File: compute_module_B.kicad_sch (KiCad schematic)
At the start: 2 parts, among them J12 HDMI_A_1.4

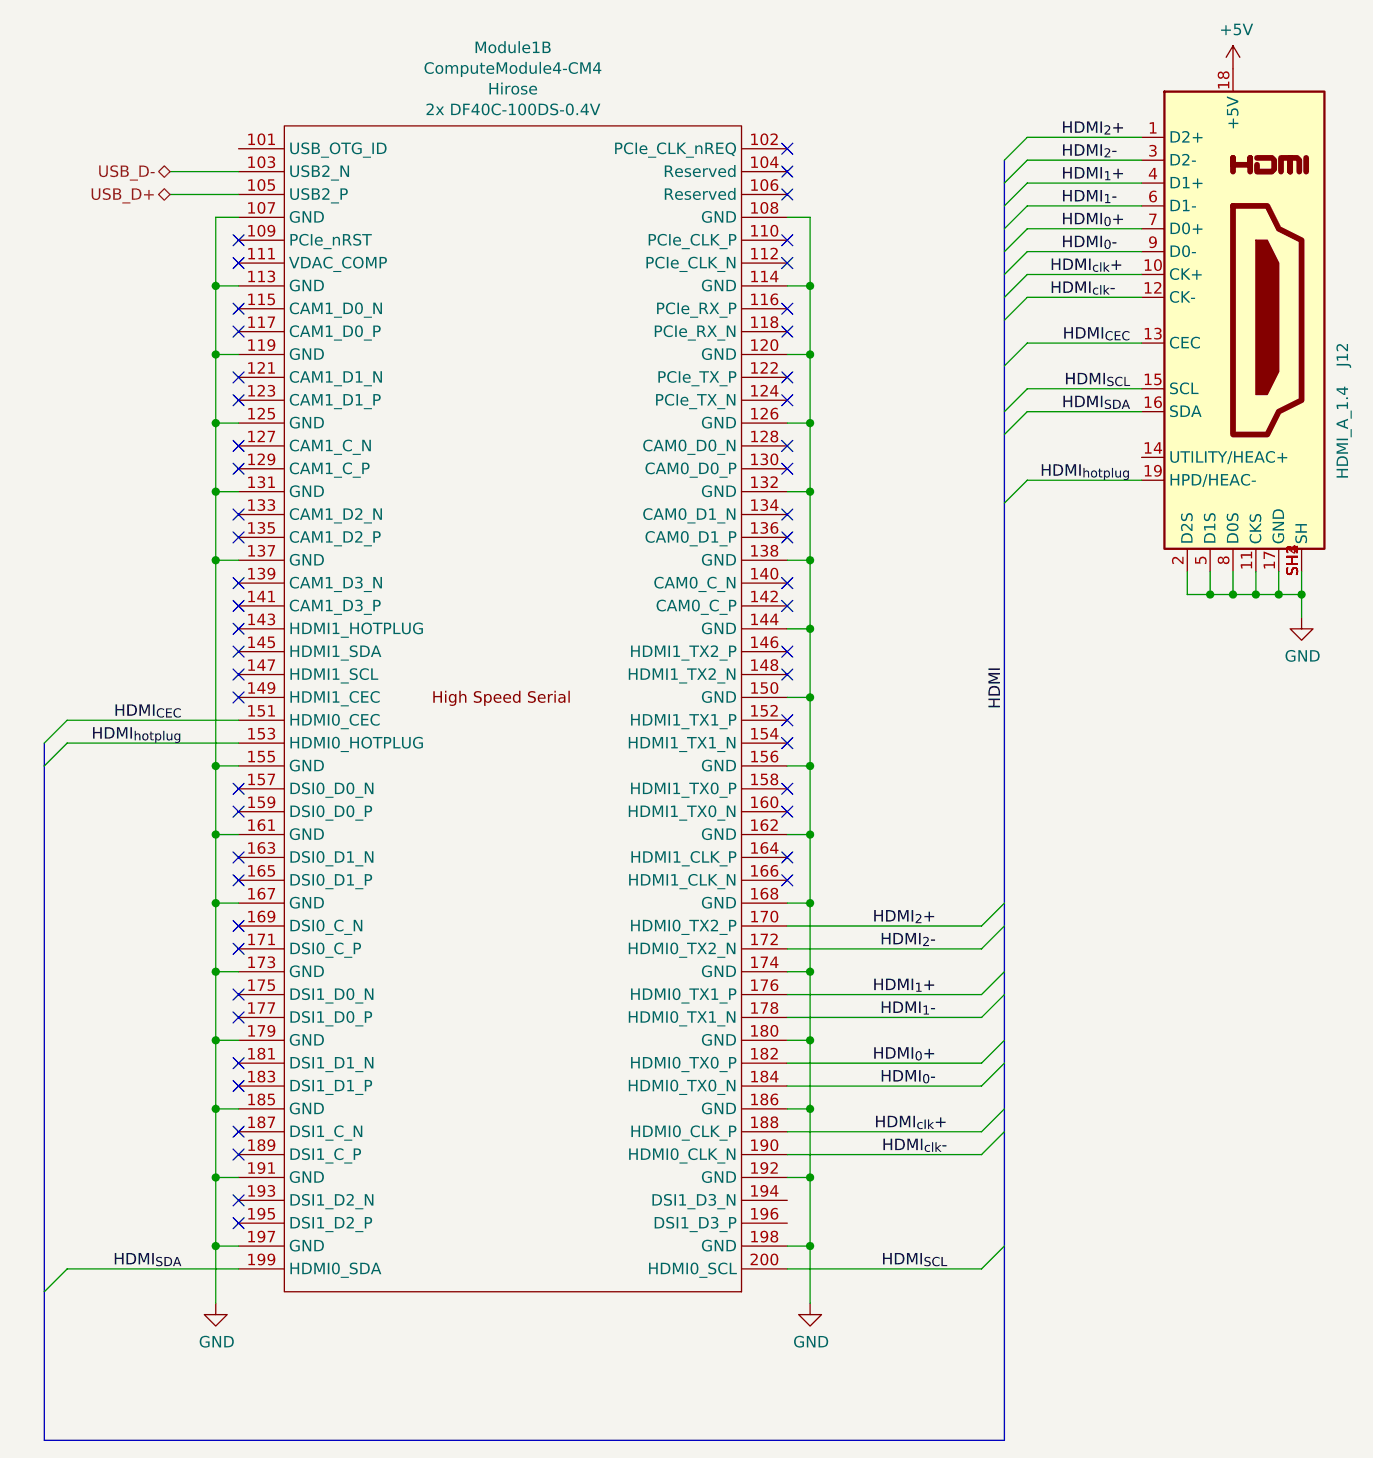
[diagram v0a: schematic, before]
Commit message: migrated computers
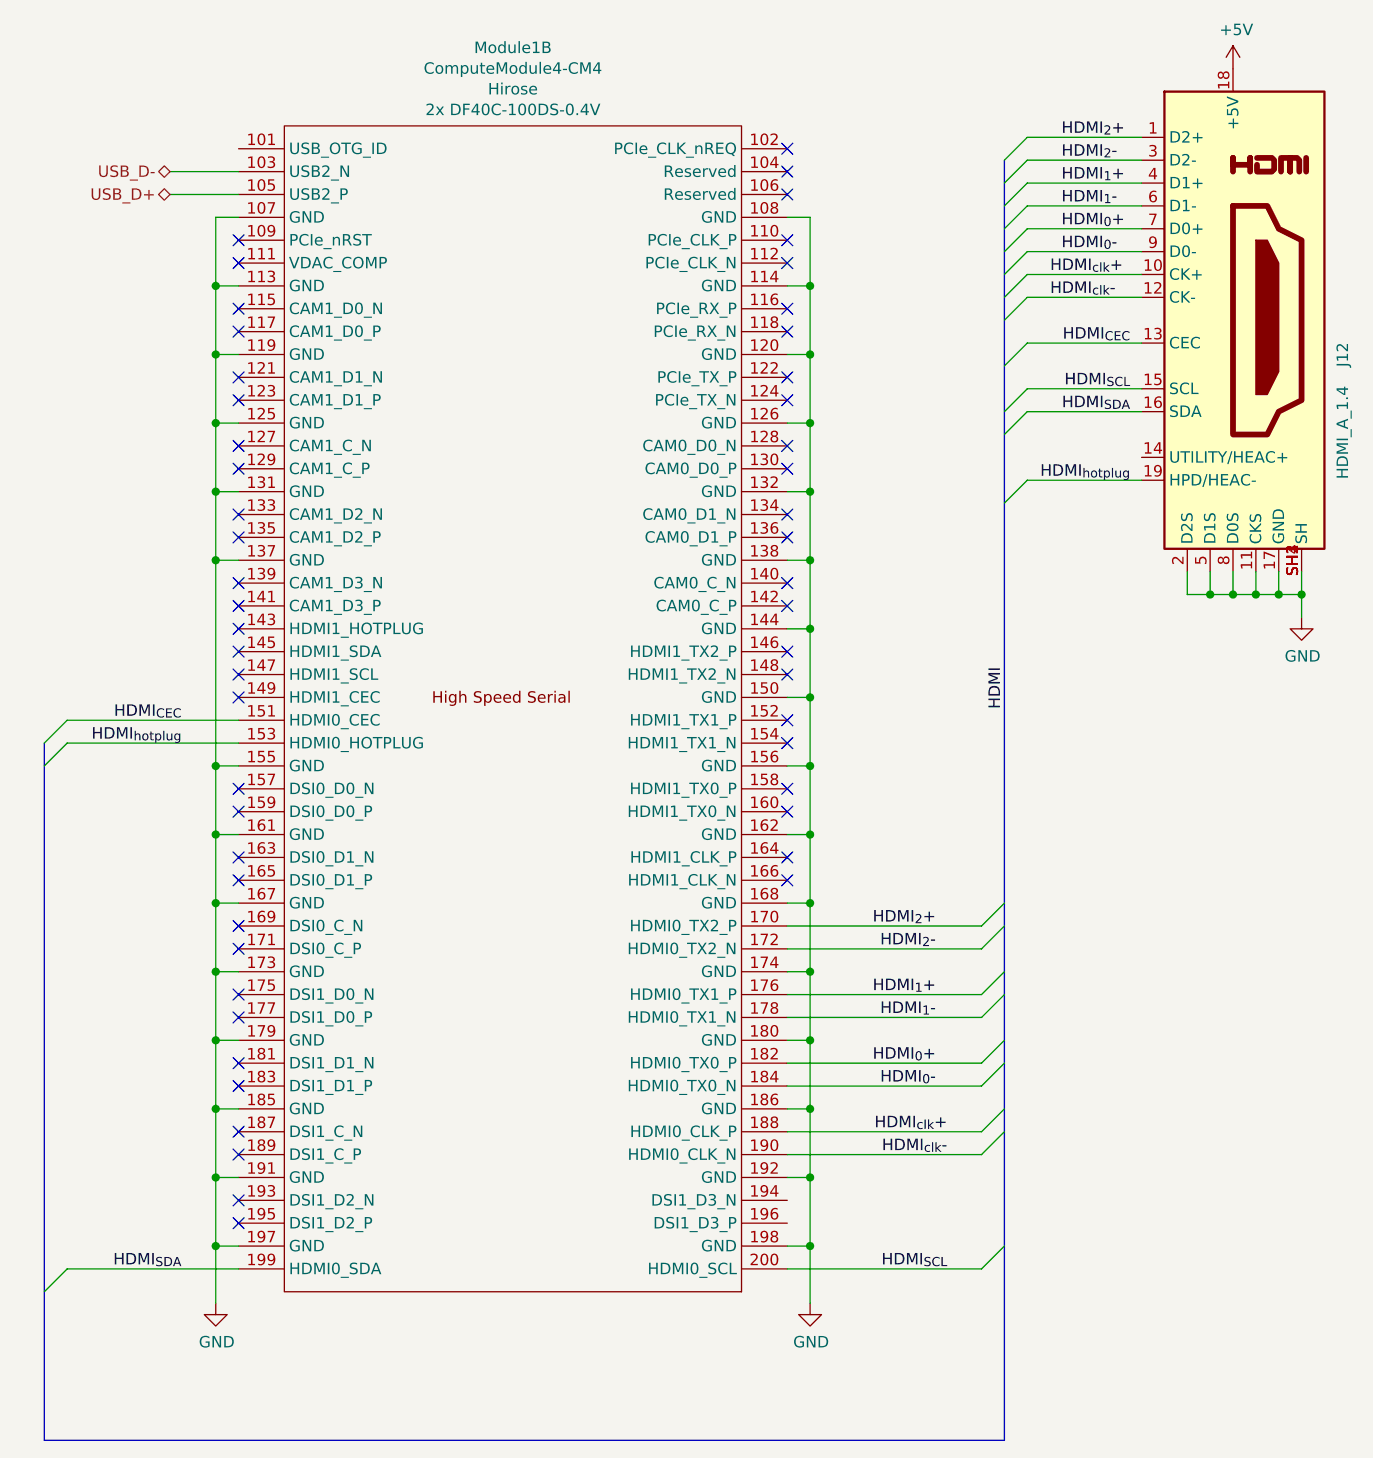
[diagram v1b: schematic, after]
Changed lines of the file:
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@@
-(kicad_sch (version 20201015) (generator eeschema)
+(kicad_sch (version 20210621) (generator eeschema)
   (paper "A")
   (title_block
@@
   (junction (at 176.53 90.17) (diameter 0.9144) (color 0 0 0 0))
   (junction (at 179.07 90.17) (diameter 0.9144) (color 0 0 0 0))
+  (no_connect (at 60.96 50.8))
+  (no_connect (at 60.96 53.34))
+  (no_connect (at 60.96 58.42))
+  (no_connect (at 60.96 60.96))
+  (no_connect (at 60.96 66.04))
+  (no_connect (at 60.96 68.58))
+  (no_connect (at 60.96 73.66))
+  (no_connect (at 60.96 76.2))
+  (no_connect (at 60.96 81.28))
+  (no_connect (at 60.96 83.82))
+  (no_connect (at 60.96 88.9))
+  (no_connect (at 60.96 91.44))
+  (no_connect (at 60.96 93.98))
+  (no_connect (at 60.96 96.52))
+  (no_connect (at 60.96 99.06))
+  (no_connect (at 60.96 101.6))
+  (no_connect (at 60.96 111.76))
+  (no_connect (at 60.96 114.3))
+  (no_connect (at 60.96 119.38))
+  (no_connect (at 60.96 121.92))
+  (no_connect (at 60.96 127))
+  (no_connect (at 60.96 129.54))
+  (no_connect (at 60.96 134.62))
+  (no_connect (at 60.96 137.16))
   (no_connect (at 60.96 142.24))
+  (no_connect (at 60.96 144.78))
+  (no_connect (at 60.96 149.86))
+  (no_connect (at 60.96 152.4))
+  (no_connect (at 60.96 157.48))
+  (no_connect (at 60.96 160.02))
+  (no_connect (at 121.92 40.64))
+  (no_connect (at 121.92 43.18))
+  (no_connect (at 121.92 45.72))
+  (no_connect (at 121.92 50.8))
+  (no_connect (at 121.92 53.34))
+  (no_connect (at 121.92 58.42))
+  (no_connect (at 121.92 60.96))
+  (no_connect (at 121.92 66.04))
+  (no_connect (at 121.92 68.58))
+  (no_connect (at 121.92 73.66))
+  (no_connect (at 121.92 76.2))
+  (no_connect (at 121.92 81.28))
+  (no_connect (at 121.92 83.82))
+  (no_connect (at 121.92 88.9))
+  (no_connect (at 121.92 91.44))
+  (no_connect (at 121.92 96.52))
   (no_connect (at 121.92 99.06))
-  (no_connect (at 121.92 60.96))
-  (no_connect (at 60.96 114.3))
-  (no_connect (at 60.96 152.4))
-  (no_connect (at 60.96 101.6))
-  (no_connect (at 121.92 96.52))
-  (no_connect (at 121.92 88.9))
-  (no_connect (at 121.92 50.8))
-  (no_connect (at 60.96 53.34))
-  (no_connect (at 121.92 40.64))
-  (no_connect (at 121.92 81.28))
-  (no_connect (at 60.96 119.38))
+  (no_connect (at 121.92 104.14))
   (no_connect (at 121.92 106.68))
-  (no_connect (at 60.96 149.86))
-  (no_connect (at 121.92 68.58))
-  (no_connect (at 60.96 129.54))
-  (no_connect (at 60.96 91.44))
-  (no_connect (at 60.96 99.06))
+  (no_connect (at 121.92 111.76))
+  (no_connect (at 121.92 114.3))
   (no_connect (at 121.92 119.38))
-  (no_connect (at 60.96 60.96))
-  (no_connect (at 121.92 114.3))
-  (no_connect (at 121.92 104.14))
-  (no_connect (at 121.92 45.72))
-  (no_connect (at 121.92 91.44))
-  (no_connect (at 60.96 83.82))
-  (no_connect (at 60.96 81.28))
-  (no_connect (at 60.96 73.66))
-  (no_connect (at 60.96 121.92))
-  (no_connect (at 121.92 111.76))
-  (no_connect (at 60.96 68.58))
-  (no_connect (at 60.96 88.9))
-  (no_connect (at 60.96 157.48))
-  (no_connect (at 60.96 134.62))
-  (no_connect (at 121.92 76.2))
-  (no_connect (at 121.92 73.66))
-  (no_connect (at 121.92 43.18))
   (no_connect (at 121.92 121.92))
-  (no_connect (at 60.96 111.76))
-  (no_connect (at 60.96 66.04))
-  (no_connect (at 121.92 66.04))
-  (no_connect (at 121.92 58.42))
-  (no_connect (at 60.96 58.42))
-  (no_connect (at 121.92 83.82))
-  (no_connect (at 60.96 137.16))
-  (no_connect (at 60.96 50.8))
-  (no_connect (at 60.96 127))
-  (no_connect (at 60.96 160.02))
-  (no_connect (at 60.96 96.52))
-  (no_connect (at 60.96 144.78))
-  (no_connect (at 121.92 53.34))
-  (no_connect (at 60.96 76.2))
-  (no_connect (at 60.96 93.98))
   (bus_entry (at 39.37 106.68) (size 2.54 -2.54)
     (stroke (width 0.1524) (type solid) (color 0 0 0 0))
@@
     (stroke (width 0) (type solid) (color 0 0 0 0))
   )
-  (bus (pts (xy 39.37 106.68) (xy 39.37 109.22))
-    (stroke (width 0) (type solid) (color 0 0 0 0))
-  )
-  (bus (pts (xy 39.37 109.22) (xy 39.37 167.64))
-    (stroke (width 0) (type solid) (color 0 0 0 0))
-  )
-  (bus (pts (xy 39.37 167.64) (xy 39.37 184.15))
+  (bus (pts (xy 39.37 106.68) (xy 39.37 184.15))
     (stroke (width 0) (type solid) (color 0 0 0 0))
   )
@@
     (stroke (width 0) (type solid) (color 0 0 0 0))
   )
-  (bus (pts (xy 146.05 41.91) (xy 146.05 44.45))
-    (stroke (width 0) (type solid) (color 0 0 0 0))
-  )
-  (bus (pts (xy 146.05 44.45) (xy 146.05 46.99))
-    (stroke (width 0) (type solid) (color 0 0 0 0))
-  )
-  (bus (pts (xy 146.05 46.99) (xy 146.05 49.53))
-    (stroke (width 0) (type solid) (color 0 0 0 0))
-  )
-  (bus (pts (xy 146.05 49.53) (xy 146.05 52.07))
-    (stroke (width 0) (type solid) (color 0 0 0 0))
-  )
-  (bus (pts (xy 146.05 52.07) (xy 146.05 54.61))
-    (stroke (width 0) (type solid) (color 0 0 0 0))
-  )
-  (bus (pts (xy 146.05 54.61) (xy 146.05 57.15))
-    (stroke (width 0) (type solid) (color 0 0 0 0))
-  )
-  (bus (pts (xy 146.05 57.15) (xy 146.05 59.69))
-    (stroke (width 0) (type solid) (color 0 0 0 0))
-  )
-  (bus (pts (xy 146.05 59.69) (xy 146.05 64.77))
-    (stroke (width 0) (type solid) (color 0 0 0 0))
-  )
-  (bus (pts (xy 146.05 64.77) (xy 146.05 69.85))
-    (stroke (width 0) (type solid) (color 0 0 0 0))
-  )
-  (bus (pts (xy 146.05 69.85) (xy 146.05 72.39))
-    (stroke (width 0) (type solid) (color 0 0 0 0))
-  )
-  (bus (pts (xy 146.05 72.39) (xy 146.05 80.01))
-    (stroke (width 0) (type solid) (color 0 0 0 0))
-  )
-  (bus (pts (xy 146.05 80.01) (xy 146.05 124.46))
-    (stroke (width 0) (type solid) (color 0 0 0 0))
-  )
-  (bus (pts (xy 146.05 124.46) (xy 146.05 127))
-    (stroke (width 0) (type solid) (color 0 0 0 0))
-  )
-  (bus (pts (xy 146.05 127) (xy 146.05 132.08))
-    (stroke (width 0) (type solid) (color 0 0 0 0))
-  )
-  (bus (pts (xy 146.05 132.08) (xy 146.05 134.62))
-    (stroke (width 0) (type solid) (color 0 0 0 0))
-  )
-  (bus (pts (xy 146.05 134.62) (xy 146.05 139.7))
-    (stroke (width 0) (type solid) (color 0 0 0 0))
-  )
-  (bus (pts (xy 146.05 139.7) (xy 146.05 142.24))
-    (stroke (width 0) (type solid) (color 0 0 0 0))
-  )
-  (bus (pts (xy 146.05 142.24) (xy 146.05 147.32))
-    (stroke (width 0) (type solid) (color 0 0 0 0))
-  )
-  (bus (pts (xy 146.05 147.32) (xy 146.05 149.86))
-    (stroke (width 0) (type solid) (color 0 0 0 0))
-  )
-  (bus (pts (xy 146.05 149.86) (xy 146.05 162.56))
-    (stroke (width 0) (type solid) (color 0 0 0 0))
-  )
-  (bus (pts (xy 146.05 162.56) (xy 146.05 184.15))
+  (bus (pts (xy 146.05 41.91) (xy 146.05 184.15))
     (stroke (width 0) (type solid) (color 0 0 0 0))
   )
@@
       (effects (font (size 1.27 1.27)) hide)
     )
+    (pin "1")
   )
   (symbol (lib_id "power:GND") (at 58.42 168.91 0) (unit 1)
@@
       (effects (font (size 1.27 1.27)) hide)
     )
+    (pin "1")
   )
   (symbol (lib_id "power:GND") (at 124.46 168.91 0) (unit 1)
@@
       (effects (font (size 1.27 1.27)) hide)
     )
+    (pin "1")
   )
   (symbol (lib_id "power:GND") (at 179.07 92.71 0) (unit 1)
@@
       (effects (font (size 1.27 1.27)) hide)
     )
+    (pin "1")
   )
   (symbol (lib_id "symbols:HDMI_A_1.4") (at 171.45 59.69 0) (unit 1)
@@
       (effects (font (size 1.27 1.27)) hide)
     )
+    (pin "SH2")
+    (pin "SH3")
+    (pin "SH4")
+    (pin "1")
+    (pin "10")
+    (pin "11")
+    (pin "12")
+    (pin "13")
+    (pin "14")
+    (pin "15")
+    (pin "16")
+    (pin "17")
+    (pin "18")
+    (pin "19")
+    (pin "2")
+    (pin "3")
+    (pin "4")
+    (pin "5")
+    (pin "6")
+    (pin "7")
+    (pin "8")
+    (pin "9")
+    (pin "SH1")
   )
   (symbol (lib_id "symbols:ComputeModule4-CM4") (at 231.14 101.6 0) (mirror y) (unit 2)
@@
     (property "Field4" "Hirose" (id 4) (at 91.44 34.0168 0))
     (property "Field5" "2x DF40C-100DS-0.4V" (id 5) (at 91.44 36.3155 0))
+    (pin "101")
+    (pin "102")
+    (pin "103")
+    (pin "104")
+    (pin "105")
+    (pin "106")
+    (pin "107")
+    (pin "108")
+    (pin "109")
+    (pin "110")
+    (pin "111")
+    (pin "112")
+    (pin "113")
+    (pin "114")
+    (pin "115")
+    (pin "116")
+    (pin "117")
+    (pin "118")
+    (pin "119")
+    (pin "120")
+    (pin "121")
+    (pin "122")
+    (pin "123")
+    (pin "124")
+    (pin "125")
+    (pin "126")
+    (pin "127")
+    (pin "128")
+    (pin "129")
+    (pin "130")
+    (pin "131")
+    (pin "132")
+    (pin "133")
+    (pin "134")
+    (pin "135")
+    (pin "136")
+    (pin "137")
+    (pin "138")
+    (pin "139")
+    (pin "140")
+    (pin "141")
+    (pin "142")
+    (pin "143")
+    (pin "144")
+    (pin "145")
+    (pin "146")
+    (pin "147")
+    (pin "148")
+    (pin "149")
+    (pin "150")
+    (pin "151")
+    (pin "152")
+    (pin "153")
+    (pin "154")
+    (pin "155")
+    (pin "156")
+    (pin "157")
+    (pin "158")
+    (pin "159")
+    (pin "160")
+    (pin "161")
+    (pin "162")
+    (pin "163")
+    (pin "164")
+    (pin "165")
+    (pin "166")
+    (pin "167")
+    (pin "168")
+    (pin "169")
+    (pin "170")
+    (pin "171")
+    (pin "172")
+    (pin "173")
+    (pin "174")
+    (pin "175")
+    (pin "176")
+    (pin "177")
+    (pin "178")
+    (pin "179")
+    (pin "180")
+    (pin "181")
+    (pin "182")
+    (pin "183")
+    (pin "184")
+    (pin "185")
+    (pin "186")
+    (pin "187")
+    (pin "188")
+    (pin "189")
+    (pin "190")
+    (pin "191")
+    (pin "192")
+    (pin "193")
+    (pin "194")
+    (pin "195")
+    (pin "196")
+    (pin "197")
+    (pin "198")
+    (pin "199")
+    (pin "200")
   )
 )
